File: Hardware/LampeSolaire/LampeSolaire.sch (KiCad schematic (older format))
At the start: 50 parts, among them K1 RELAIS_DPDT, P1 1V8, P2 3V5, P3 3V5, P4 2V, T1 SI2333, T2 SI2333, T3 FDN337, T4 FDN337, T5 FDN337, T6 FDN337, T7 FDN337, U1 MCP73832, U2 MCP121, U3 NCP114ASN330T1G, U4 MRF89XAM8A, U5 PIC16F1827, U6 74xx00, X1 SOLAR_CELL, X2 ICSP, X4 BUZZER, X6 WATER_SENSOR

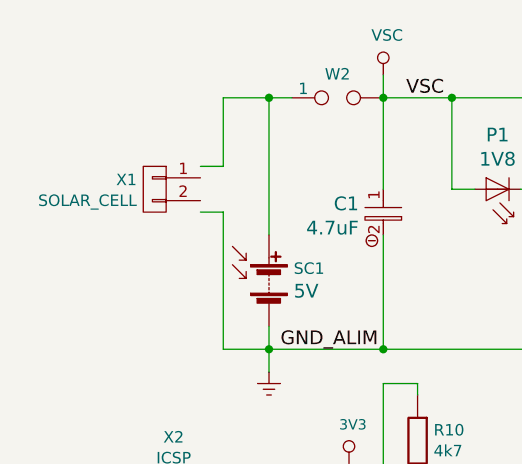
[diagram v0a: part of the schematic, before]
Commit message: V5 Complete
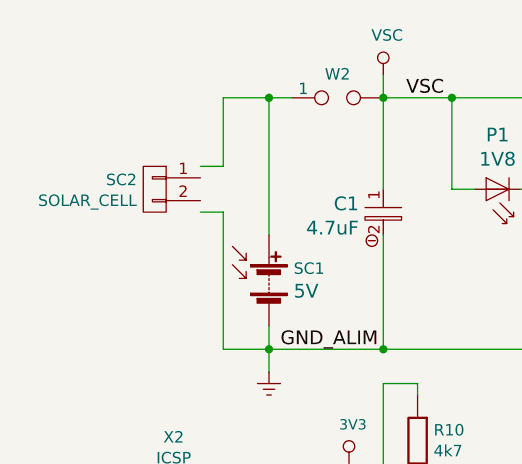
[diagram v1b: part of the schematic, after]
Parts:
- P2, P3, SC1, X4, X6: footprint 0EsseivaN_Lib:CH_2P -> 0EsseivaN_Lib:CH_02P
- SC2: renamed from X1; footprint 0EsseivaN_Lib:CH_2P -> 0EsseivaN_Lib:CH_02P
- V1: footprint 0EsseivaN_Lib:CH_3P -> 0EsseivaN_Lib:CH_03P
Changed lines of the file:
@@
 F 0 "SC1" H 1408 1753 50  0000 L CNN
 F 1 "Solar_Cells" H 1400 1700 50  0001 L CNN
-F 2 "0EsseivaN_Lib:CH_2P" V 1300 1760 50  0001 C CNN
+F 2 "0EsseivaN_Lib:CH_02P" V 1300 1760 50  0001 C CNN
 F 3 "" V 1300 1760 50  0000 C CNN
 F 4 "5V" H 1408 1654 60  0000 L CNN "Voltage"
@@
 F 0 "P2" V 9547 6022 60  0000 R CNN
 F 1 "3V5" V 9653 6022 60  0000 R CNN
-F 2 "0EsseivaN_Lib:CH_2P" H 9600 6200 60  0001 C CNN
+F 2 "0EsseivaN_Lib:CH_02P" H 9600 6200 60  0001 C CNN
 F 3 "" H 9600 6200 60  0000 C CNN
 	1    9600 6200
@@
 F 0 "P3" V 9947 6278 60  0000 L CNN
 F 1 "3V5" V 10053 6278 60  0000 L CNN
-F 2 "0EsseivaN_Lib:CH_2P" H 10000 6200 60  0001 C CNN
+F 2 "0EsseivaN_Lib:CH_02P" H 10000 6200 60  0001 C CNN
 F 3 "" H 10000 6200 60  0000 C CNN
 	1    10000 6200
@@
 $EndComp
 $Comp
-L 0EsseivaN_Lib:CONN_01X02 X1
+L 0EsseivaN_Lib:CONN_01X02 SC2
 U 1 1 5B71F5E8
 P 800 1300
-F 0 "X1" H 878 1341 50  0000 L CNN
+F 0 "SC2" H 878 1341 50  0000 L CNN
 F 1 "SOLAR_CELL" H 878 1250 50  0000 L CNN
-F 2 "0EsseivaN_Lib:CH_2P" H 800 1250 50  0001 C CNN
+F 2 "0EsseivaN_Lib:CH_02P" H 800 1250 50  0001 C CNN
 F 3 "" H 800 1250 50  0000 C CNN
 	1    800  1300
@@
 F 0 "X4" H 4117 2715 50  0000 C CNN
 F 1 "BUZZER" H 4117 2624 50  0000 C CNN
-F 2 "0EsseivaN_Lib:CH_2P" H 4200 2350 50  0001 C CNN
+F 2 "0EsseivaN_Lib:CH_02P" H 4200 2350 50  0001 C CNN
 F 3 "" H 4200 2350 50  0000 C CNN
 	1    4200 2400
@@
 F 0 "V1" H 5450 1950 60  0000 C CNN
 F 1 "Li battery" H 5600 1850 60  0000 C CNN
-F 2 "0EsseivaN_Lib:CH_3P" H 5310 1750 60  0001 C CNN
+F 2 "0EsseivaN_Lib:CH_03P" H 5310 1750 60  0001 C CNN
 F 3 "" H 5310 1750 60  0001 C CNN
 F 4 "3V7" H 5500 1550 60  0000 C CNN "Voltage"
@@
 F 0 "X6" H 7628 2691 50  0000 L CNN
 F 1 "WATER_SENSOR" H 7628 2600 50  0000 L CNN
-F 2 "0EsseivaN_Lib:CH_2P" H 7550 2600 50  0001 C CNN
+F 2 "0EsseivaN_Lib:CH_02P" H 7550 2600 50  0001 C CNN
 F 3 "" H 7550 2600 50  0000 C CNN
 	1    7550 2650
